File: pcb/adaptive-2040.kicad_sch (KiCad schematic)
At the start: 20 parts, among them J1 USB_A, J10 AudioJack2, J11 AudioJack2, J12 AudioJack2, J13 AudioJack2, J14 AudioJack2, J15 AudioJack2, J16 AudioJack2, J17 AudioJack2, J18 AudioJack2, J19 AudioJack2, J2 AudioJack2, J3 AudioJack2, J4 AudioJack2, J5 AudioJack2, J6 AudioJack2, J7 AudioJack2, J8 AudioJack2, J9 AudioJack2, U1 RaspberryPi_Pico

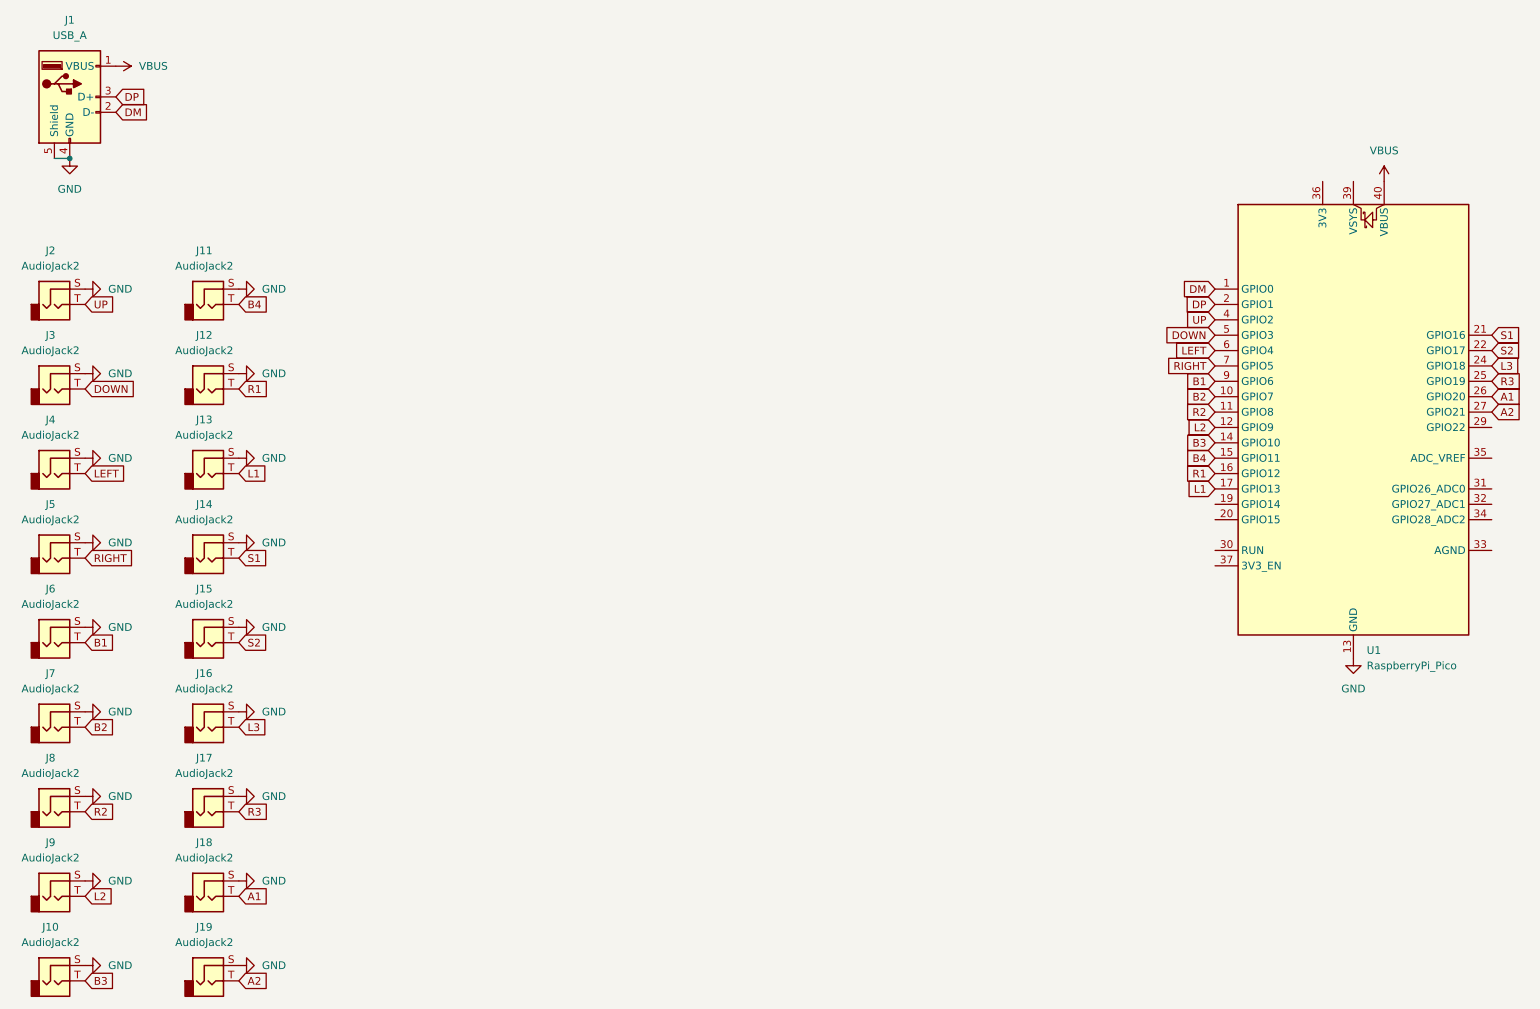
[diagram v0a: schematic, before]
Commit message: tidy things up a little
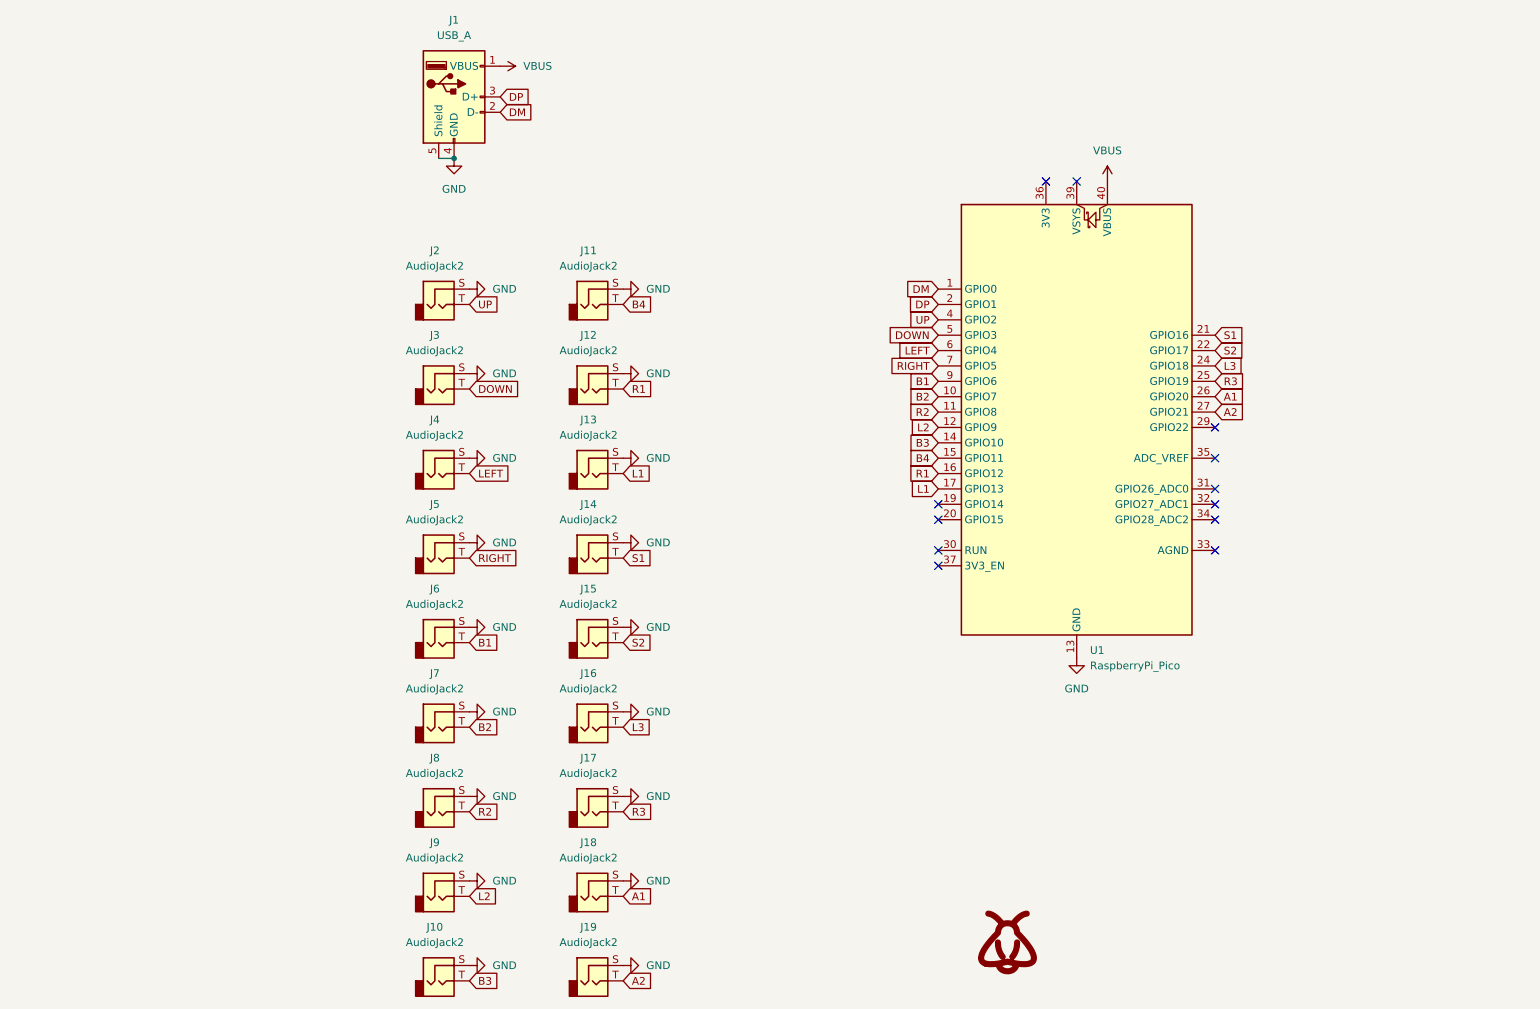
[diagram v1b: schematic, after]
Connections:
- no-connect marks 0 -> 12
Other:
- company: (none) -> moth.monster
- title: (none) -> adaptive2040
- moved on the sheet: J1, J10, J11, J12, J13, J14, J15, J16, J17, J18, J19, J2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
